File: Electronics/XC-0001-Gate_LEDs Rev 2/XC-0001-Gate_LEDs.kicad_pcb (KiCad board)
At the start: 2 copper layers, 76 x 60 mm, 16 parts, among them J1 DC12V_IN, J2 BuckBlock_NP, J3 LED_DIM, J4 LED_NODIM, J5 AC_IN, J6 AC_OUT

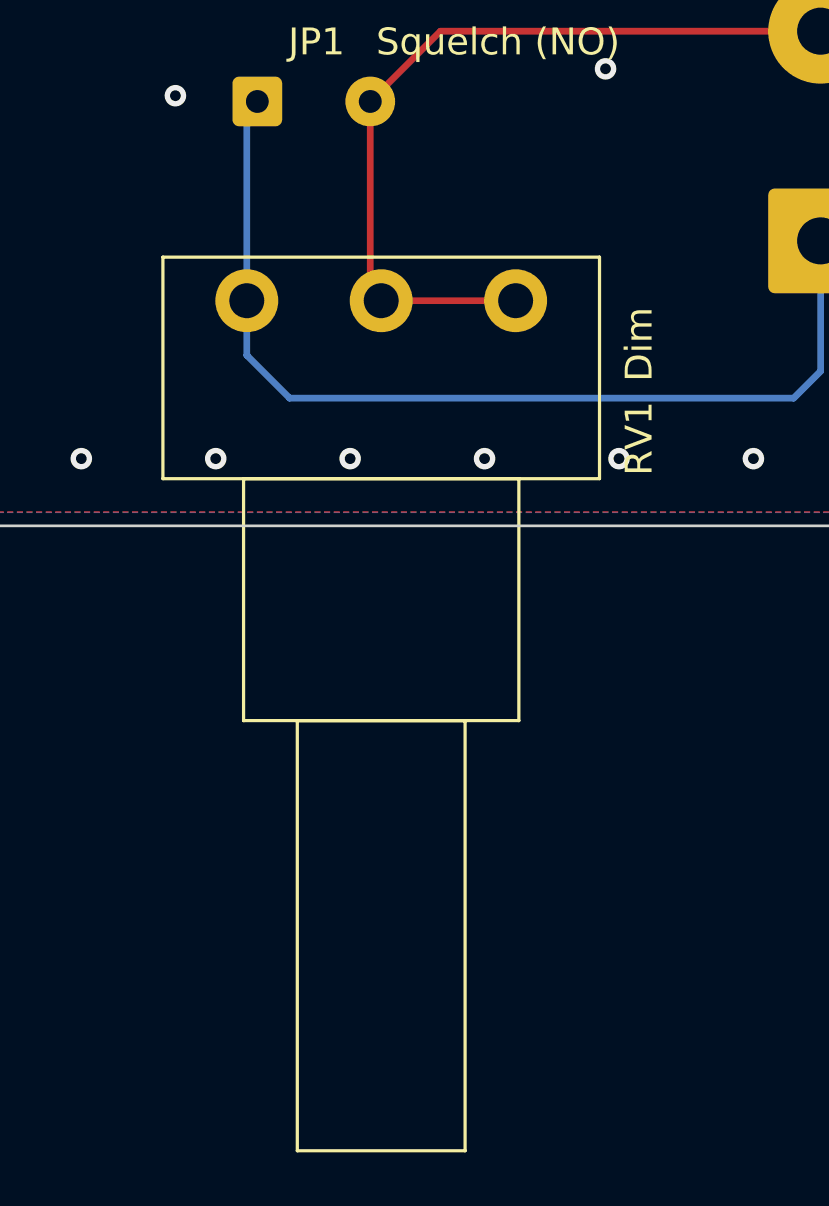
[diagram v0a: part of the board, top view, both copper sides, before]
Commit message: Version 2 updates
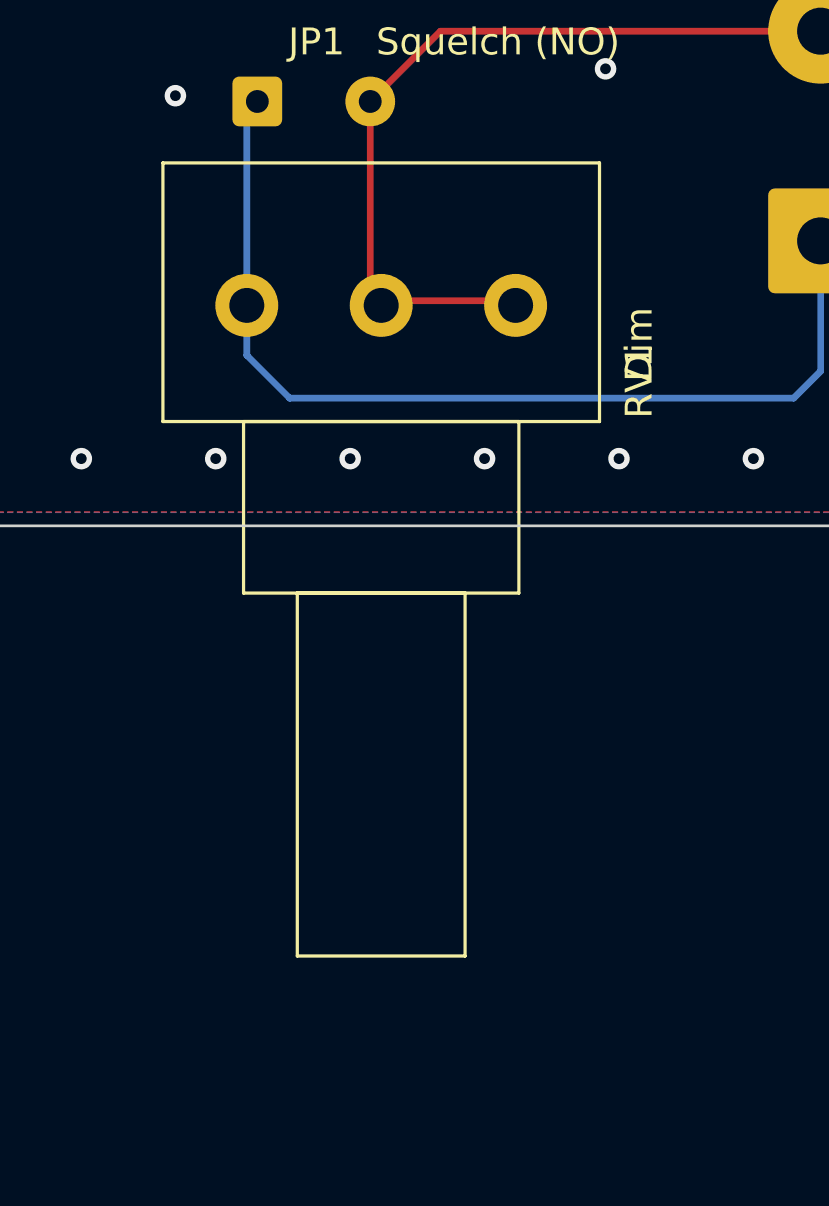
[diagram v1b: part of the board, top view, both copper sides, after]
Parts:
- RV1: footprint Potentiometer_THT:Potentiometer_Piher_PC-16_Single_Horizontal -> XC-footprint-lib:Potentiometer_Bourns_PDB181-K420K-203B
- moved RV1 2.13 mm to (118.7, 119.5)
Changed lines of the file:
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@@
   )
   (setup
-    (last_trace_width 0.6)
+    (last_trace_width 0.25)
     (user_trace_width 0.25)
     (user_trace_width 0.6)
@@
     (add_net DC-12V)
   )
+  (module XC-footprint-lib:Potentiometer_Bourns_PDB181-K420K-203B (layer F.Cu)
+    (at 118.655531 119.5 270)
+    (descr "Potentiometer, horizontal, Piher PC-16 Single, http://www.piher-nacesa.com/pdf/20-PC16v03.pdf")
+    (tags "Potentiometer horizontal Piher PC-16 Single")
+    (fp_text reference RV1 (at 5.12489 -14.594469 90) (layer F.SilkS)
+      (effects (font (size 1 1) (thickness 0.15)))
+    )
+    (fp_text value DIM_POT (at 0 4.25 90) (layer F.Fab)
+      (effects (font (size 1 1) (thickness 0.15)))
+    )
+    (fp_line (start 26.7 -13.25) (end -3.2 -13.25) (layer F.CrtYd) (width 0.05))
+    (fp_line (start 26.7 3.25) (end 26.7 -13.25) (layer F.CrtYd) (width 0.05))
+    (fp_line (start -3.2 3.25) (end 26.7 3.25) (layer F.CrtYd) (width 0.05))
+    (fp_line (start -3.2 -13.25) (end -3.2 3.25) (layer F.CrtYd) (width 0.05))
+    (fp_line (start 26.5 -8.12) (end 26.5 -1.879) (layer F.SilkS) (width 0.12))
+    (fp_line (start 13 -8.12) (end 13 -1.879) (layer F.SilkS) (width 0.12))
+    (fp_line (start 13 -1.879) (end 26.5 -1.879) (layer F.SilkS) (width 0.12))
+    (fp_line (start 13 -8.12) (end 26.5 -8.12) (layer F.SilkS) (width 0.12))
+    (fp_line (start 13 -10.12) (end 13 0.12) (layer F.SilkS) (width 0.12))
+    (fp_line (start 6.62 -10.12) (end 6.62 0.12) (layer F.SilkS) (width 0.12))
+    (fp_line (start 6.62 0.12) (end 13 0.12) (layer F.SilkS) (width 0.12))
+    (fp_line (start 6.62 -10.12) (end 13 -10.12) (layer F.SilkS) (width 0.12))
+    (fp_line (start 6.62 -13.12) (end 6.62 3.12) (layer F.SilkS) (width 0.12))
+    (fp_line (start -3 -13.12) (end -3 3.12) (layer F.SilkS) (width 0.12))
+    (fp_line (start -3 3.12) (end 6.62 3.12) (layer F.SilkS) (width 0.12))
+    (fp_line (start -3 -13.12) (end 6.62 -13.12) (layer F.SilkS) (width 0.12))
+    (fp_line (start 26.3 -8) (end 12.9 -8) (layer F.Fab) (width 0.1))
+    (fp_line (start 26.3 -2) (end 26.3 -8) (layer F.Fab) (width 0.1))
+    (fp_line (start 12.9 -2) (end 26.3 -2) (layer F.Fab) (width 0.1))
+    (fp_line (start 12.9 -8.1) (end 12.9 -2.1) (layer F.Fab) (width 0.1))
+    (fp_line (start 12.8 -10) (end 6.5 -10) (layer F.Fab) (width 0.1))
+    (fp_line (start 12.9 0) (end 12.9 -10) (layer F.Fab) (width 0.1))
+    (fp_line (start 6.5 0) (end 12.9 0) (layer F.Fab) (width 0.1))
+    (fp_line (start 6.5 -10) (end 6.5 0) (layer F.Fab) (width 0.1))
+    (fp_line (start 6.5 -13) (end -2.9 -13) (layer F.Fab) (width 0.1))
+    (fp_line (start 6.5 3) (end 6.5 -13) (layer F.Fab) (width 0.1))
+    (fp_line (start -2.8 3) (end 6.5 3) (layer F.Fab) (width 0.1))
+    (fp_line (start -2.9 -13) (end -2.9 3) (layer F.Fab) (width 0.1))
+    (fp_text user %R (at 9.654999 2.264999 90) (layer F.Fab)
+      (effects (font (size 1 1) (thickness 0.15)))
+    )
+    (pad 1 thru_hole circle (at 2.3 0 270) (size 2.34 2.34) (drill 1.3) (layers *.Cu *.Mask)
+      (net 1 /DIM_GND))
+    (pad 2 thru_hole circle (at 2.3 -5 270) (size 2.34 2.34) (drill 1.3) (layers *.Cu *.Mask)
+      (net 7 /DIM_ANALOG))
+    (pad 3 thru_hole circle (at 2.3 -10 270) (size 2.34 2.34) (drill 1.3) (layers *.Cu *.Mask)
+      (net 7 /DIM_ANALOG))
+    (model C:/Users/james/Dev/homeprojects/Electronics/Parts/PDB181-K420K.stp
+      (offset (xyz 6.24 4.9784 12.7))
+      (scale (xyz 1 1 1))
+      (rotate (xyz -90 0 0))
+    )
+  )
   (module Diode_THT:D_T-1_P10.16mm_Horizontal (layer F.Cu)
     (at 91.75 112.5 180)
@@
     (fp_text value DIODE (at 5.08 2.42) (layer F.Fab)
       (effects (font (size 1 1) (thickness 0.15)))
-    )
-    (fp_text user K (at 0 -2) (layer F.SilkS)
-      (effects (font (size 1 1) (thickness 0.15)))
-    )
-    (fp_text user K (at 0 -2) (layer F.Fab)
-      (effects (font (size 1 1) (thickness 0.15)))
-    )
-    (fp_text user %R (at 5.32 0) (layer F.Fab)
-      (effects (font (size 0.64 0.64) (thickness 0.096)))
     )
     (fp_line (start 3.48 -1.3) (end 3.48 1.3) (layer F.Fab) (width 0.1))
@@
     (fp_line (start 11.41 1.55) (end 11.41 -1.55) (layer F.CrtYd) (width 0.05))
     (fp_line (start 11.41 -1.55) (end -1.25 -1.55) (layer F.CrtYd) (width 0.05))
+    (fp_text user K (at 0 -2) (layer F.SilkS)
+      (effects (font (size 1 1) (thickness 0.15)))
+    )
+    (fp_text user K (at 0 -2) (layer F.Fab)
+      (effects (font (size 1 1) (thickness 0.15)))
+    )
+    (fp_text user %R (at 5.32 0) (layer F.Fab)
+      (effects (font (size 0.64 0.64) (thickness 0.096)))
+    )
     (pad 1 thru_hole oval (at 10.16 0 180) (size 2 2) (drill 1) (layers *.Cu *.Mask)
       (net 4 NEUT))
@@
       (at (xyz 0 0 0))
       (scale (xyz 1 1 1))
-      (rotate (xyz 0 0 0))
-    )
-  )
-  (module Potentiometer_THT:Potentiometer_Piher_PC-16_Single_Horizontal (layer F.Cu)
-    (at 118.655531 121.62511 270)
-    (descr "Potentiometer, horizontal, Piher PC-16 Single, http://www.piher-nacesa.com/pdf/20-PC16v03.pdf")
-    (tags "Potentiometer horizontal Piher PC-16 Single")
-    (fp_text reference RV1 (at 5.12489 -14.594469 90) (layer F.SilkS)
-      (effects (font (size 1 1) (thickness 0.15)))
-    )
-    (fp_text value DIM_POT (at 0 4.25 90) (layer F.Fab)
-      (effects (font (size 1 1) (thickness 0.15)))
-    )
-    (fp_line (start 31.75 -13.25) (end -1.75 -13.25) (layer F.CrtYd) (width 0.05))
-    (fp_line (start 31.75 3.25) (end 31.75 -13.25) (layer F.CrtYd) (width 0.05))
-    (fp_line (start -1.75 3.25) (end 31.75 3.25) (layer F.CrtYd) (width 0.05))
-    (fp_line (start -1.75 -13.25) (end -1.75 3.25) (layer F.CrtYd) (width 0.05))
-    (fp_line (start 31.62 -8.12) (end 31.62 -1.879) (layer F.SilkS) (width 0.12))
-    (fp_line (start 15.62 -8.12) (end 15.62 -1.879) (layer F.SilkS) (width 0.12))
-    (fp_line (start 15.62 -1.879) (end 31.62 -1.879) (layer F.SilkS) (width 0.12))
-    (fp_line (start 15.62 -8.12) (end 31.62 -8.12) (layer F.SilkS) (width 0.12))
-    (fp_line (start 15.62 -10.12) (end 15.62 0.12) (layer F.SilkS) (width 0.12))
-    (fp_line (start 6.62 -10.12) (end 6.62 0.12) (layer F.SilkS) (width 0.12))
-    (fp_line (start 6.62 0.12) (end 15.62 0.12) (layer F.SilkS) (width 0.12))
-    (fp_line (start 6.62 -10.12) (end 15.62 -10.12) (layer F.SilkS) (width 0.12))
-    (fp_line (start 6.62 -13.12) (end 6.62 3.12) (layer F.SilkS) (width 0.12))
-    (fp_line (start -1.62 -13.12) (end -1.62 3.12) (layer F.SilkS) (width 0.12))
-    (fp_line (start -1.62 3.12) (end 6.62 3.12) (layer F.SilkS) (width 0.12))
-    (fp_line (start -1.62 -13.12) (end 6.62 -13.12) (layer F.SilkS) (width 0.12))
-    (fp_line (start 31.5 -8) (end 15.5 -8) (layer F.Fab) (width 0.1))
-    (fp_line (start 31.5 -2) (end 31.5 -8) (layer F.Fab) (width 0.1))
-    (fp_line (start 15.5 -2) (end 31.5 -2) (layer F.Fab) (width 0.1))
-    (fp_line (start 15.5 -8) (end 15.5 -2) (layer F.Fab) (width 0.1))
-    (fp_line (start 15.5 -10) (end 6.5 -10) (layer F.Fab) (width 0.1))
-    (fp_line (start 15.5 0) (end 15.5 -10) (layer F.Fab) (width 0.1))
-    (fp_line (start 6.5 0) (end 15.5 0) (layer F.Fab) (width 0.1))
-    (fp_line (start 6.5 -10) (end 6.5 0) (layer F.Fab) (width 0.1))
-    (fp_line (start 6.5 -13) (end -1.5 -13) (layer F.Fab) (width 0.1))
-    (fp_line (start 6.5 3) (end 6.5 -13) (layer F.Fab) (width 0.1))
-    (fp_line (start -1.5 3) (end 6.5 3) (layer F.Fab) (width 0.1))
-    (fp_line (start -1.5 -13) (end -1.5 3) (layer F.Fab) (width 0.1))
-    (fp_text user %R (at 9.654999 2.264999 90) (layer F.Fab)
-      (effects (font (size 1 1) (thickness 0.15)))
-    )
-    (pad 3 thru_hole circle (at 0 -10 270) (size 2.34 2.34) (drill 1.3) (layers *.Cu *.Mask)
-      (net 7 /DIM_ANALOG))
-    (pad 2 thru_hole circle (at 0 -5 270) (size 2.34 2.34) (drill 1.3) (layers *.Cu *.Mask)
-      (net 7 /DIM_ANALOG))
-    (pad 1 thru_hole circle (at 0 0 270) (size 2.34 2.34) (drill 1.3) (layers *.Cu *.Mask)
-      (net 1 /DIM_GND))
-    (model ${KISYS3DMOD}/Potentiometer_THT.3dshapes/Potentiometer_Piher_PC-16_Single_Horizontal.wrl
-      (at (xyz 0 0 0))
-      (scale (xyz 1 1 1))

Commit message: Update to KiCAD 7.x, bump Rev. to 2a (not manufactured)
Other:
- net class AC removed
- net class DC Pwr removed
- net class Default removed
